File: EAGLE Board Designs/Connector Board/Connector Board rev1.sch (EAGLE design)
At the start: 14 parts, among them J1 CONNECTOR-37__, J2 CONNECTOR-8_AMPHENOL_M12A_08P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, J3 CONNECTOR-8_AMPHENOL_M12A_08P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, J4 CONNECTOR-6_AS_PCT_, J5 CONNECTOR-13_SOURIAU_, J6 CONNECTOR-40__, J7 CONNECTOR-40__

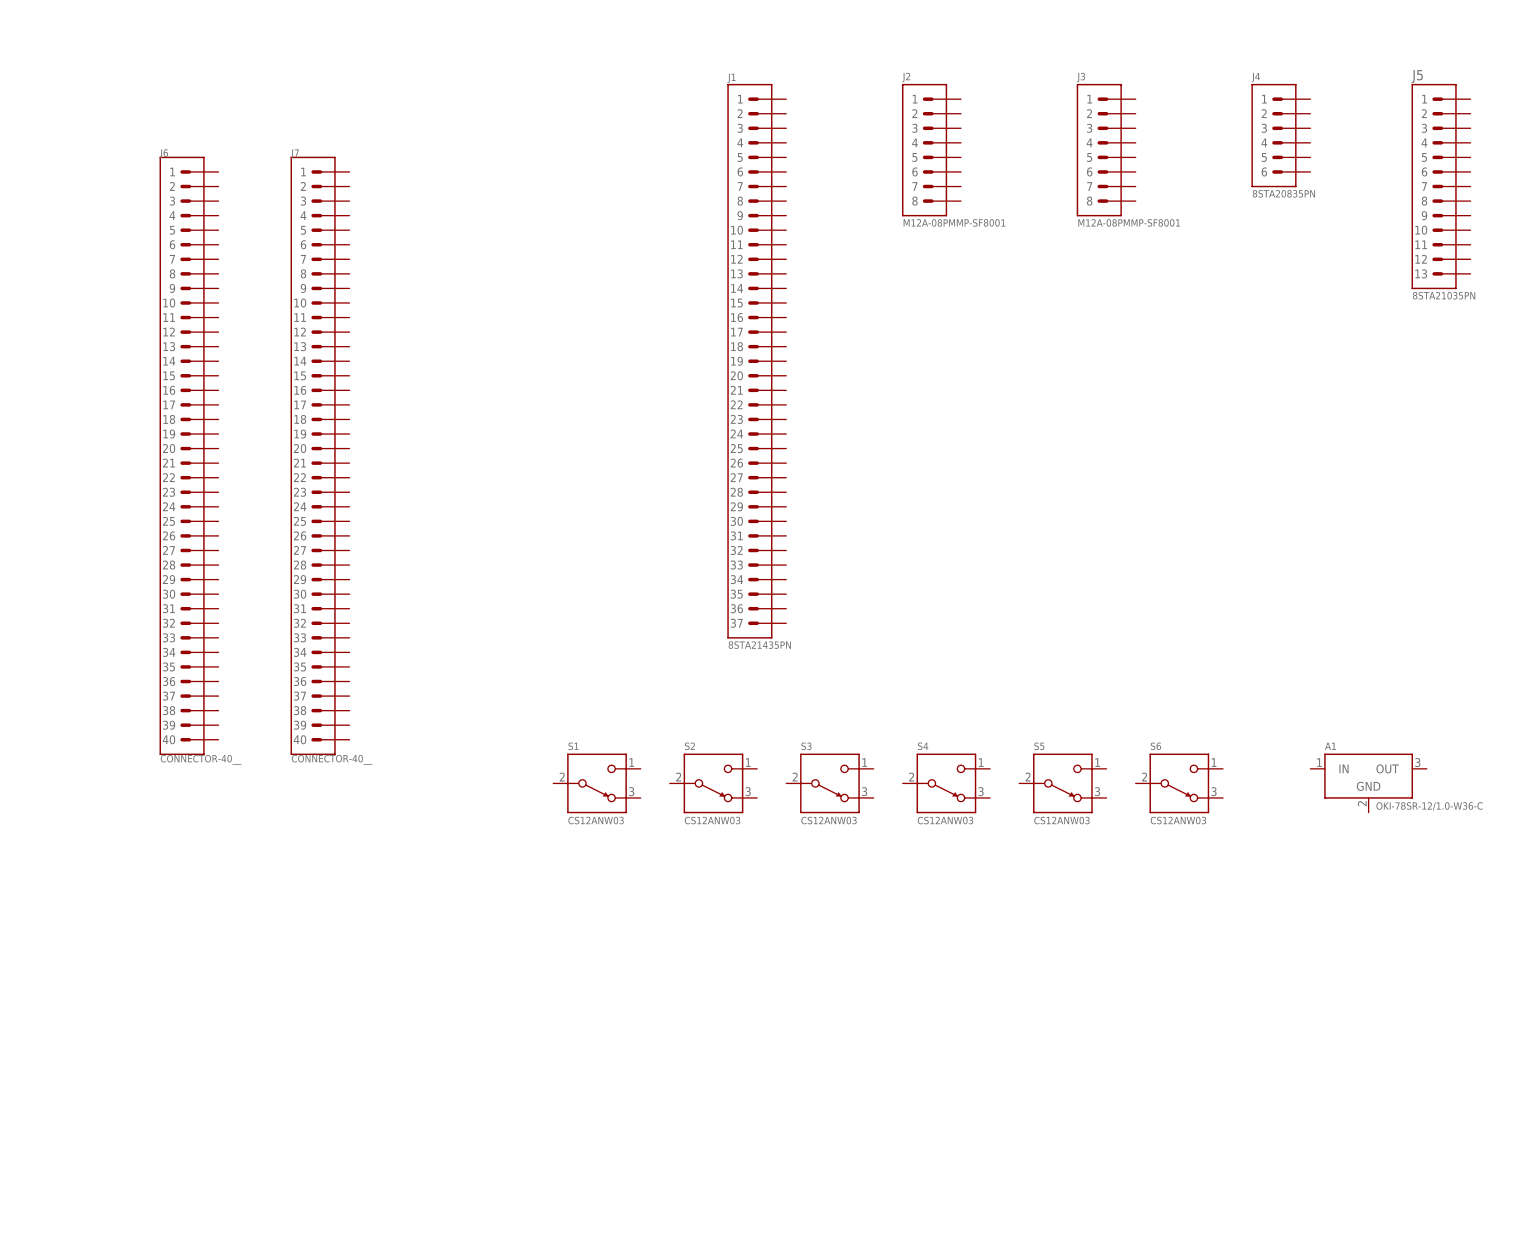
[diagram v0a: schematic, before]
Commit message: some definitions
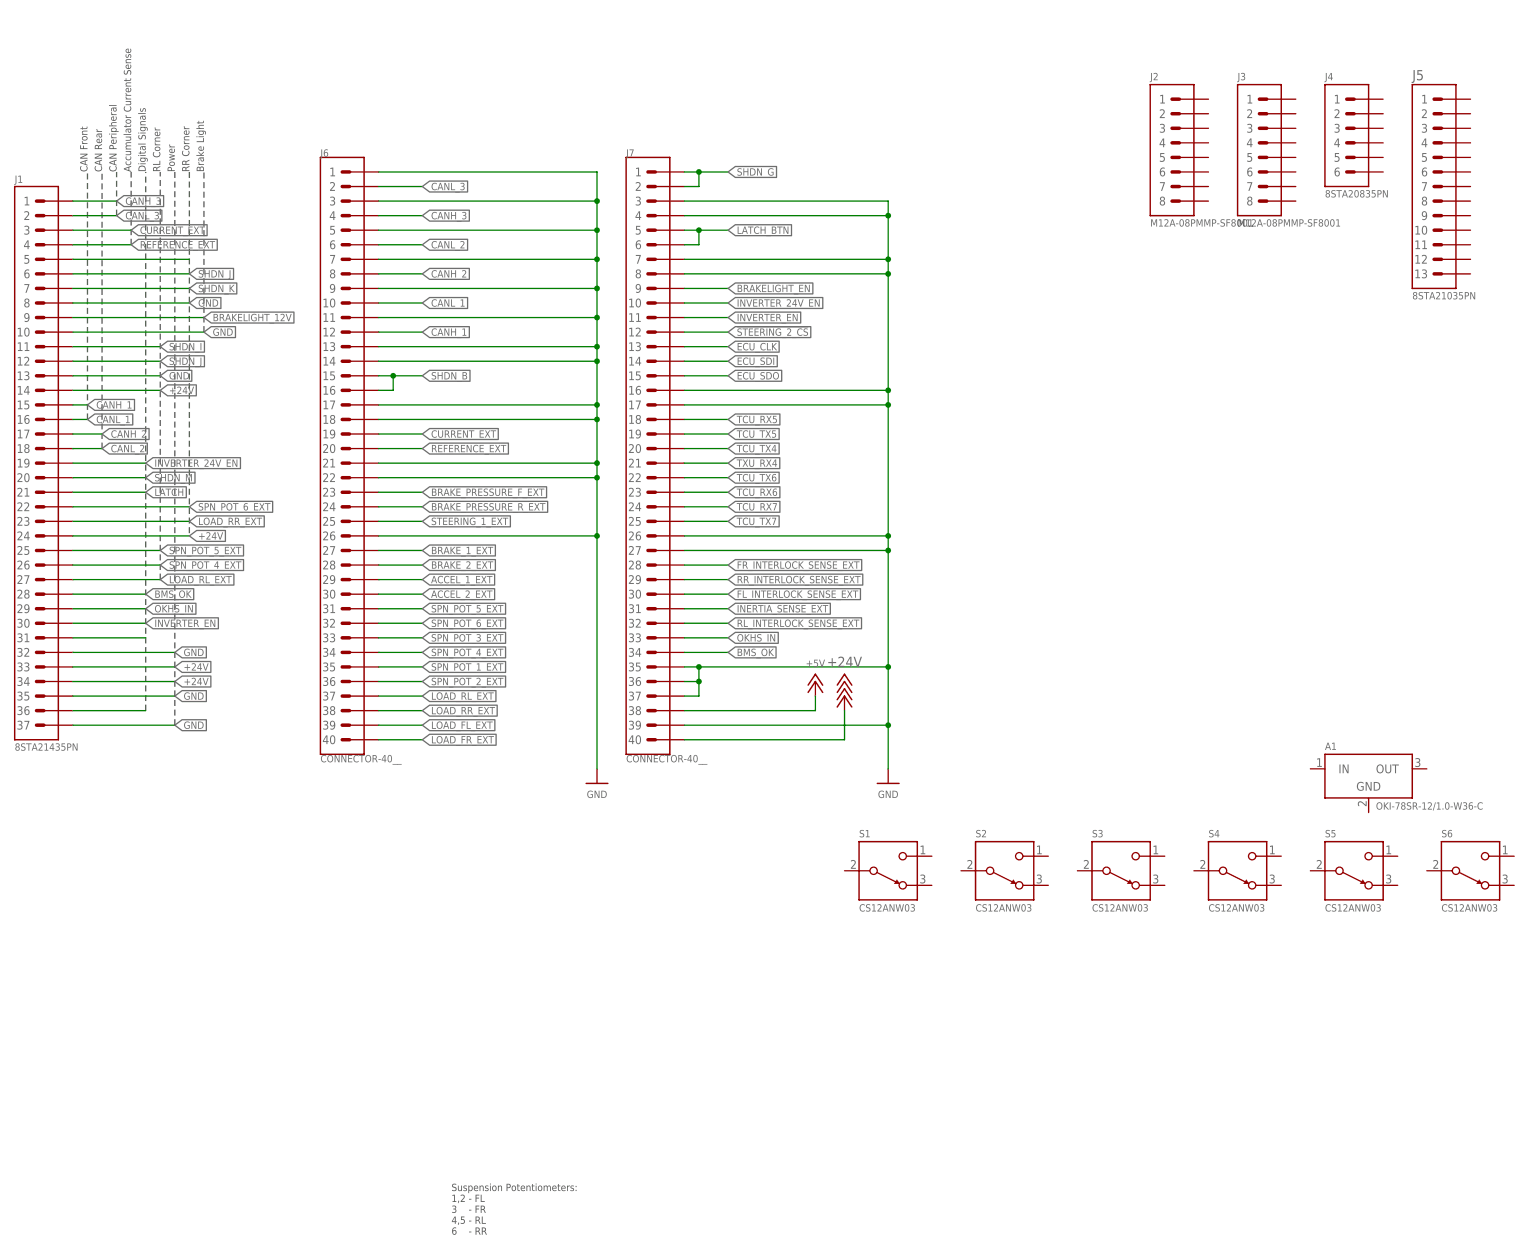
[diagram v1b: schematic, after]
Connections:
- new net !STEERING_2_CS: J7.12
- new net +24V: J1.14, J1.24, J1.33, J1.34, J7.40
- new net +5V: J7.38
- new net ACCEL_1_EXT: J6.29
- new net ACCEL_2_EXT: J6.30
- new net BMS_OK: J1.28, J7.34
- new net BRAKELIGHT_12V: J1.9
- new net BRAKELIGHT_EN: J7.9
- new net BRAKE_1_EXT: J6.27
- new net BRAKE_2_EXT: J6.28
- new net BRAKE_PRESSURE_F_EXT: J6.23
- new net BRAKE_PRESSURE_R_EXT: J6.24
- new net CANH_1: J1.15, J6.12
- new net CANH_2: J1.17, J6.8
- new net CANH_3: J1.1, J6.4
- new net CANL_1: J1.16, J6.10
- new net CANL_2: J1.18, J6.6
- new net CANL_3: J1.2, J6.2
- new net CURRENT_EXT: J1.3, J6.19
- new net ECU_CLK: J7.13
- new net ECU_SDI: J7.14
- new net ECU_SDO: J7.15
- new net FL_INTERLOCK_SENSE_EXT: J7.30
- new net FR_INTERLOCK_SENSE_EXT: J7.28
- new net GND: J1.10, J1.13, J1.32, J1.35, J1.37, J1.8, J6.1, J6.11, J6.13, J6.14, J6.17, J6.18, J6.21, J6.22, J6.26, J6.3, J6.5, J6.7, J6.9, J7.16, J7.17, J7.26, J7.27, J7.3, J7.35, J7.36, J7.37, J7.39, J7.4, J7.7, J7.8
- new net INERTIA_SENSE_EXT: J7.31
- new net INVERTER_24V_EN: J1.19, J7.10
- new net INVERTER_EN: J1.30, J7.11
- new net LATCH: J1.21
- new net LATCH_BTN: J7.5, J7.6
- new net LOAD_FL_EXT: J6.39
- new net LOAD_FR_EXT: J6.40
- new net LOAD_RL_EXT: J1.27, J6.37
- new net LOAD_RR_EXT: J1.23, J6.38
- new net N$1: J1.5
- new net N$4: J1.31
- new net N$5: J1.36
- new net OKHS_IN: J1.29, J7.33
- new net REFERENCE_EXT: J1.4, J6.20
- new net RL_INTERLOCK_SENSE_EXT: J7.32
- new net RR_INTERLOCK_SENSE_EXT: J7.29
- new net SHDN_B: J6.15, J6.16
- new net SHDN_G: J7.1, J7.2
- new net SHDN_I: J1.11
- new net SHDN_J: J1.12, J1.6
- new net SHDN_K: J1.7
- new net SHDN_M: J1.20
- new net SPN_POT_1_EXT: J6.35
- new net SPN_POT_2_EXT: J6.36
- new net SPN_POT_3_EXT: J6.33
- new net SPN_POT_4_EXT: J1.26, J6.34
- new net SPN_POT_5_EXT: J1.25, J6.31
- new net SPN_POT_6_EXT: J1.22, J6.32
- new net STEERING_1_EXT: J6.25
- new net TCU_RX5: J7.18
- new net TCU_RX6: J7.23
- new net TCU_RX7: J7.24
- new net TCU_TX4: J7.20
- new net TCU_TX5: J7.19
- new net TCU_TX6: J7.22
- new net TCU_TX7: J7.25
- new net TXU_RX4: J7.21
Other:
- note added: "Accumulator Current Sense"
- note added: "Brake Light"
- note added: "CAN Front"
- note added: "CAN Peripheral"
- note added: "CAN Rear"
- note added: "Digital Signals"
- note added: "Power"
- note added: "RL Corner"
- note added: "RR Corner"
- note added: "Suspension Potentiometers: 1,2 - FL 3 - FR 4,5 - RL 6 - RR"
- moved on the sheet: J1, J2, J3, J4, J6, J7, S1, S2, S3, S4, S5, S6
